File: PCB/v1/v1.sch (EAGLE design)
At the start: 69 parts, among them U2 AT24C512C-SHD-B

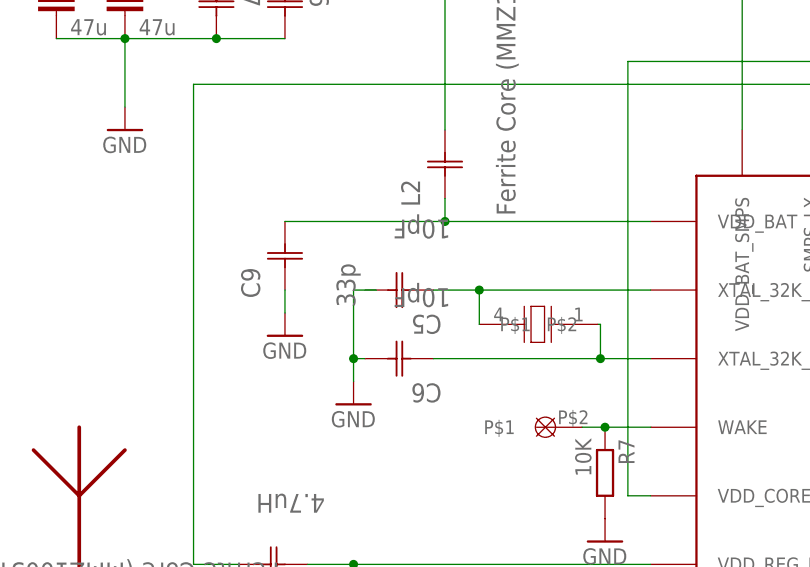
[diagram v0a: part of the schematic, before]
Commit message: submitting for fabrication
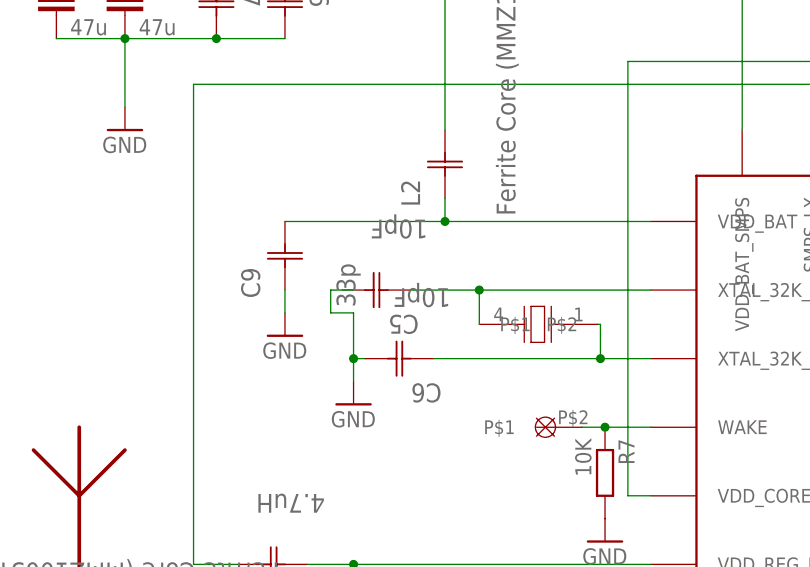
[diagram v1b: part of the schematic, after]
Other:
- moved on the sheet: C5
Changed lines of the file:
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@@
 <instance part="C3" gate="A" x="-91.44" y="0" rot="R90"/>
 <instance part="C4" gate="A" x="-76.2" y="0" rot="R90"/>
-<instance part="C5" gate="A" x="-120.65" y="73.66" rot="R180"/>
+<instance part="C5" gate="A" x="-123.19" y="73.66" rot="R180"/>
 <instance part="C6" gate="A" x="-120.65" y="66.04" rot="R180"/>
 <instance part="GND3" gate="1" x="-83.82" y="-7.366"/>
@@
 <pinref part="C6" gate="A" pin="C2"/>
 <wire x1="-128.27" y1="66.04" x2="-129.54" y2="66.04" width="0.1524" layer="91"/>
-<wire x1="-129.54" y1="66.04" x2="-129.54" y2="73.66" width="0.1524" layer="91"/>
+<wire x1="-129.54" y1="66.04" x2="-129.54" y2="71.12" width="0.1524" layer="91"/>
 <junction x="-129.54" y="66.04"/>
-<wire x1="-127" y1="73.66" x2="-129.54" y2="73.66" width="0.1524" layer="91"/>
+<wire x1="-129.54" y1="71.12" x2="-132.08" y2="71.12" width="0.1524" layer="91"/>
+<wire x1="-132.08" y1="71.12" x2="-132.08" y2="73.66" width="0.1524" layer="91"/>
+<wire x1="-132.08" y1="73.66" x2="-129.54" y2="73.66" width="0.1524" layer="91"/>
 </segment>
 <segment>
@@
 <segment>
 <pinref part="C5" gate="A" pin="C1"/>
-<wire x1="-120.65" y1="73.66" x2="-115.57" y2="73.66" width="0.1524" layer="91"/>
+<wire x1="-123.19" y1="73.66" x2="-115.57" y2="73.66" width="0.1524" layer="91"/>
 <pinref part="U$4" gate="G$1" pin="P$2"/>
 <wire x1="-115.57" y1="73.66" x2="-96.52" y2="73.66" width="0.1524" layer="91"/>
